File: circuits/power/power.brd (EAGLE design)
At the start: 26.6 x 13.7 mm, 22 parts

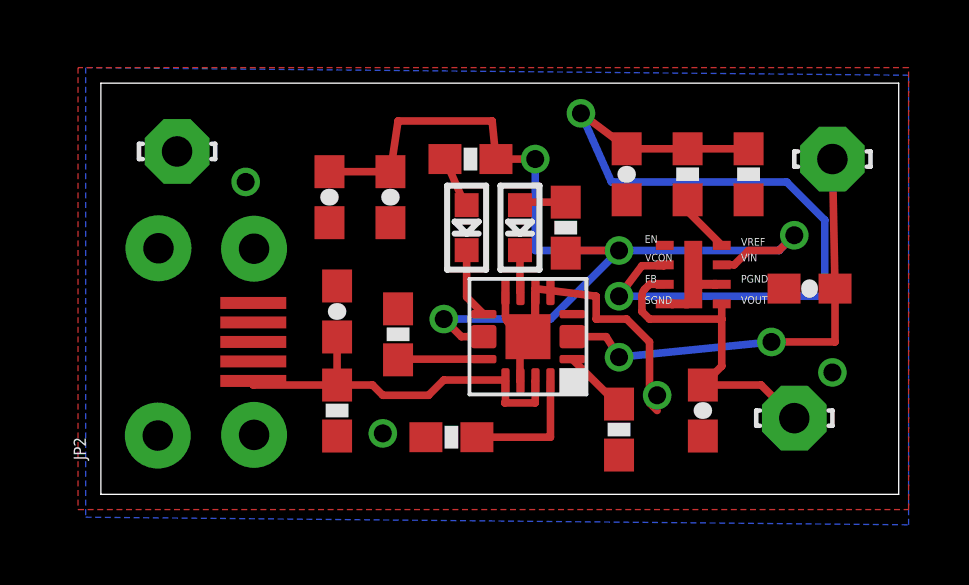
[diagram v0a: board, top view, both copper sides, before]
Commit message: stuff I dont know
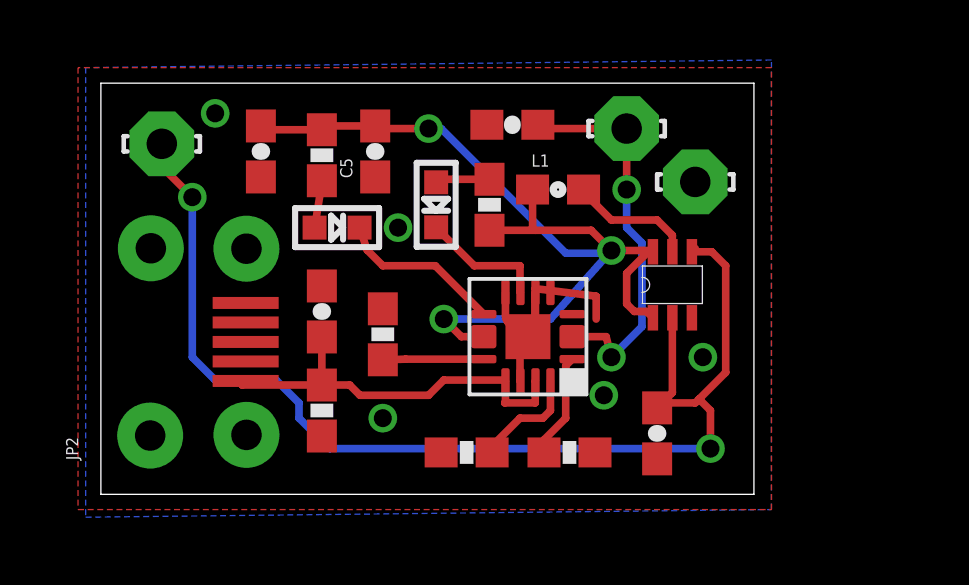
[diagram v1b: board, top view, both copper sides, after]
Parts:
- removed C6: 470pF, SparkFun-Capacitors:0603-CAP
- removed R7: 118k, SparkFun-Passives:0603-RES
- removed R8: 150k, SparkFun-Passives:0603-RES
- removed U$2: LMZ10500, LMZ10500:LMZ10500
- added L1: 10uH, SparkFun-Passives:0603
- added U$3: TLV61225, tps6122x:SC70
- moved LSP3 23.0 mm to (2.03, 11.7)
- moved LSP1 17.3 mm to (19.8, 10.4)
- moved C2 11.3 mm to (13.7, 12.3)
- moved LSP2 6.93 mm to (17.5, 12.2)
- moved R5 4.95 mm to (7.37, 11.3), turned to 270 degrees
- moved LED2 4.32 mm to (7.87, 8.89), turned to 270 degrees
- moved LED1 2.90 mm to (11.2, 9.65)
- moved C1 2.75 mm to (5.33, 11.4)
- moved R4 2.65 mm to (13.0, 9.65)
- moved R3 1.82 mm to (15.6, 1.40), turned to 180 degrees
- moved C4 1.70 mm to (18.5, 2.03)
- moved C5 1.61 mm to (9.14, 11.4)
- moved R2 0.72 mm to (12.2, 1.40)
- moved R1 0.51 mm to (9.40, 5.33)
- moved C3 0.51 mm to (7.37, 6.10)
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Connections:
- removed net N$2: C6.1, R7.1, R8.2, U$2.VCON
- net GND: no longer C6.2, R8.1, U$2.PGND, U$2.SGND
- net N$1: now also L1.2, U$3.L; no longer R7.2, U$2.VREF
- net N$9: now also L1.1, U$3.EN, U$3.VIN; no longer U$2.VIN
- net VOUT: now also U$3.FB, U$3.VOUT; no longer U$2.FB, U$2.VOUT
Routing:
- net VOUT: track 10.7 -> 39.2 mm, vias 0 -> 2
- net N$2: track 27.6 -> 0.00 mm, vias 2 -> 0
- net GND: track 13.5 -> 9.06 mm, vias 4 -> 5
- net N$12: track 2.37 -> 5.56 mm
- net N$13: track 1.42 -> 4.22 mm
- net N$1: track 1.99 -> 4.19 mm
- net BAT: track 15.3 -> 13.1 mm
- net N$9: track 34.4 -> 32.3 mm, vias 4 -> 3
- net N$6: track 2.16 -> 3.50 mm
- net N$5: track 4.33 -> 3.64 mm
- net N$3: track 2.86 -> 3.36 mm
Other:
- board size 26.6 x 13.7 mm -> 21.8 x 13.7 mm
